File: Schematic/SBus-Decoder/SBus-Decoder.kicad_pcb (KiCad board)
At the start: 2 copper layers, 10 parts, among them J1 Conn_01x03_Male, J2 Conn_01x01_Male, J3 Conn_02x03_Odd_Even, U1 PIC16F18313-I_SN, U2 MCP1703A-3302_SOT23

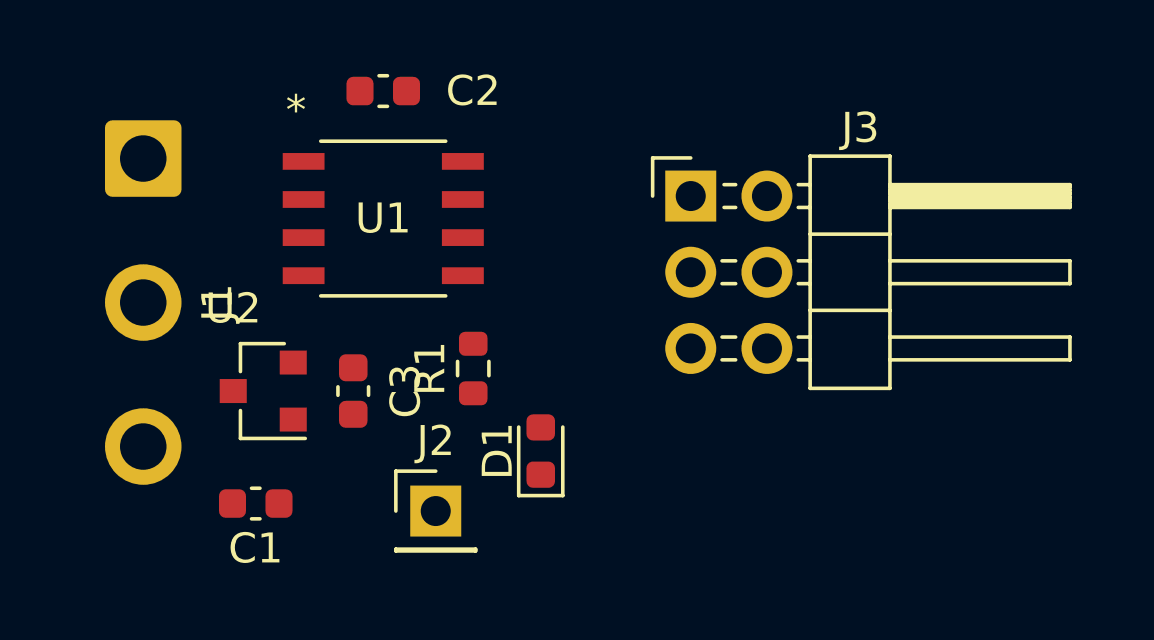
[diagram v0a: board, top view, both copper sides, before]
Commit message: Initial pcb
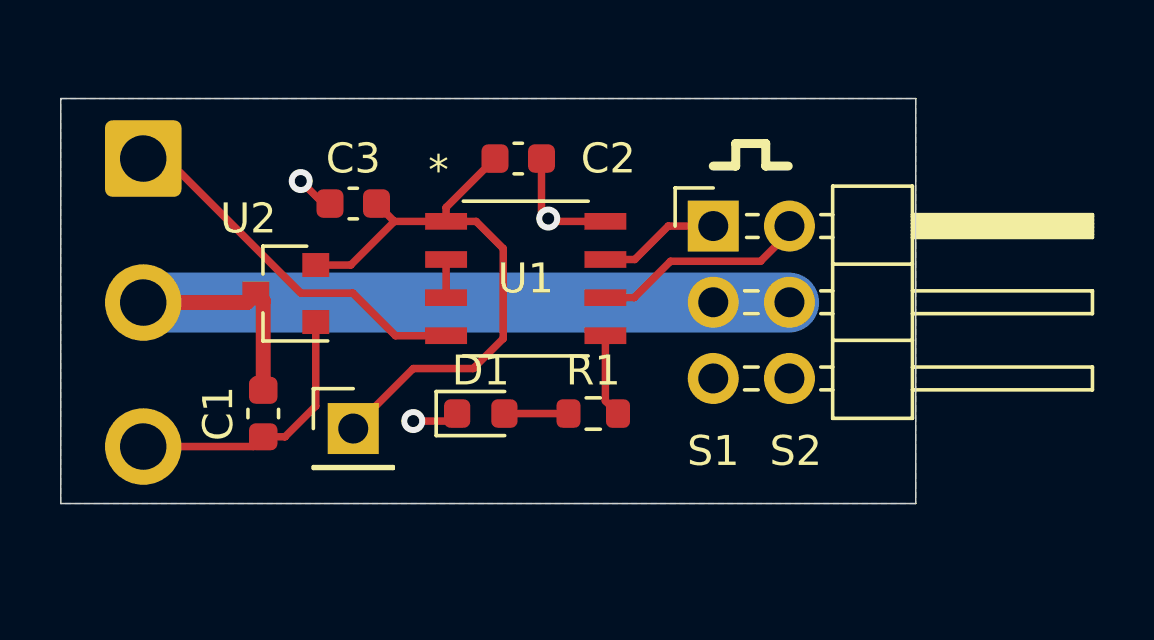
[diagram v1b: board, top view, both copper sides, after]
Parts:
- moved C3 6.25 mm to (109.8, 105.8), turned to 180 degrees
- moved U1 5.15 mm to (115.5, 108.2)
- moved C2 5.03 mm to (115.2, 104.2)
- moved R1 4.27 mm to (117.8, 112.8), turned to 0 degrees
- moved J2 3.89 mm to (109.8, 113.2)
- moved U2 3.34 mm to (107.5, 108.8)
- moved C1 3.01 mm to (106.8, 112.8), turned to 270 degrees
- moved D1 2.36 mm to (114.0, 112.8), turned to 0 degrees
- moved J3 1.25 mm to (121.8, 106.5)
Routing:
- net VBUS: track 0.00 -> 29.1 mm
- net +3V3: track 0.00 -> 20.1 mm
- net GND: track 0.00 -> 16.0 mm, vias 0 -> 3
- net Net-(J1-Pad1): track 0.00 -> 12.7 mm
- net Net-(J3-Pad2): track 0.00 -> 7.25 mm
- net Net-(J3-Pad1): track 0.00 -> 4.06 mm
- net Net-(R1-Pad2): track 0.00 -> 2.77 mm
- net Net-(D1-Pad2): track 0.00 -> 2.14 mm
- net Net-(U1-Pad2): track 0.00 -> 1.27 mm
- added copper zone on B.Cu, net GND
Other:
- board outline added: 28.5 x 13.5 mm
- net class Power: trace_width 1 -> 0.5
- board text added: "S1"
- board text added: "S2"

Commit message: Schematic and pcb
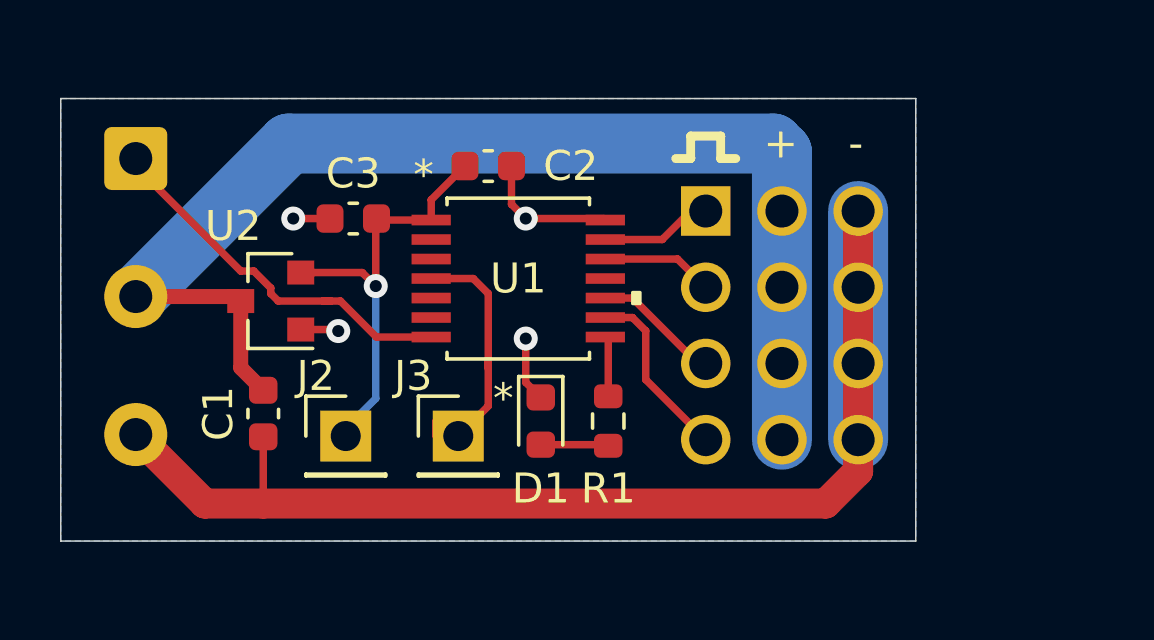
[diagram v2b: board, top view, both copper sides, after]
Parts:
- added J4: TSW-104-08-G-T-RA, SamacSys_Parts:HDRRA12W64P254_3X4_1016X254X810P, F.Cu at (121.5, 106.0)
- J1: footprint Connector_Wire:SolderWire-0.75sqmm_1x03_P4.8mm_D1.25mm_OD2.3mm -> Connector_Wire:SolderWire-0.5sqmm_1x03_P4.6mm_D0.9mm_OD2.1mm
- J3: value Conn_02x03_Odd_Even -> Conn_01x01_Male; footprint Connector_PinHeader_2.54mm:PinHeader_2x03_P2.54mm_Horizontal -> Connector_PinHeader_2.54mm:PinHeader_1x01_P2.54mm_Vertical
- U1: value PIC16F18313-I_SN -> PIC18F04Q40-I_ST; footprint PIC16F18313:PIC16F18313-I&slash_SN -> PIC18F0xQ40:PIC18F04Q40-I&slash_ST
- moved J3 11.0 mm to (113.2, 113.5)
- moved D1 2.02 mm to (116.0, 113.0), turned to 270 degrees
- moved C2 1.03 mm to (114.2, 104.5)
- moved R1 0.56 mm to (118.2, 113.0), turned to 90 degrees
- moved U2 0.56 mm to (107.0, 109.0)
- moved C3 0.50 mm to (109.8, 106.2)
- moved J2 0.35 mm to (109.5, 113.5)
- moved J1 0.25 mm to (102.5, 104.2)
- moved U1 0.25 mm to (115.2, 108.2)
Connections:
- U1 pad 3: Net-(U1-Pad2) -> Net-(U1-Pad3)
- U1 pad 4: Net-(J1-Pad1) -> Net-(J3-Pad1)
- U1 pad 5: Net-(R1-Pad2) -> Net-(U1-Pad5)
- U1 pad 6: Net-(J3-Pad2) -> Net-(U1-Pad6)
- U1 pad 7: Net-(J3-Pad1) -> Net-(J1-Pad1)
- U1 pad 8: GND -> Net-(R1-Pad2)
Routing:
- net GND: track 16.0 -> 53.4 mm, vias 3 -> 4
- net VBUS: track 29.1 -> 40.2 mm
- net Net-(J3-Pad2): track 7.25 -> 0.00 mm
- net Net-(J4-Pad10): track 0.00 -> 5.99 mm
- net +3V3: track 20.1 -> 14.9 mm, vias 0 -> 1
- net Net-(J4-Pad7): track 0.00 -> 4.25 mm
- net Net-(J3-Pad1): track 4.06 -> 8.02 mm
- net Net-(J4-Pad1): track 0.00 -> 3.74 mm
- net Net-(J4-Pad4): track 0.00 -> 3.74 mm
- net Net-(U1-Pad2): track 1.27 -> 0.00 mm
- net Net-(R1-Pad2): track 2.77 -> 2.02 mm
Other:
- board size 28.5 x 13.5 mm -> 28.5 x 14.8 mm
- board text added: "*"
- board text added: "+"
- board text added: "-"
- board text added: "SBus Decoder V1.0 QES 2021"
- board text removed: "S1"
- board text removed: "S2"
